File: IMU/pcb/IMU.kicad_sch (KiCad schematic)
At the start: 1 part, among them J2 Conn_01x10_Socket

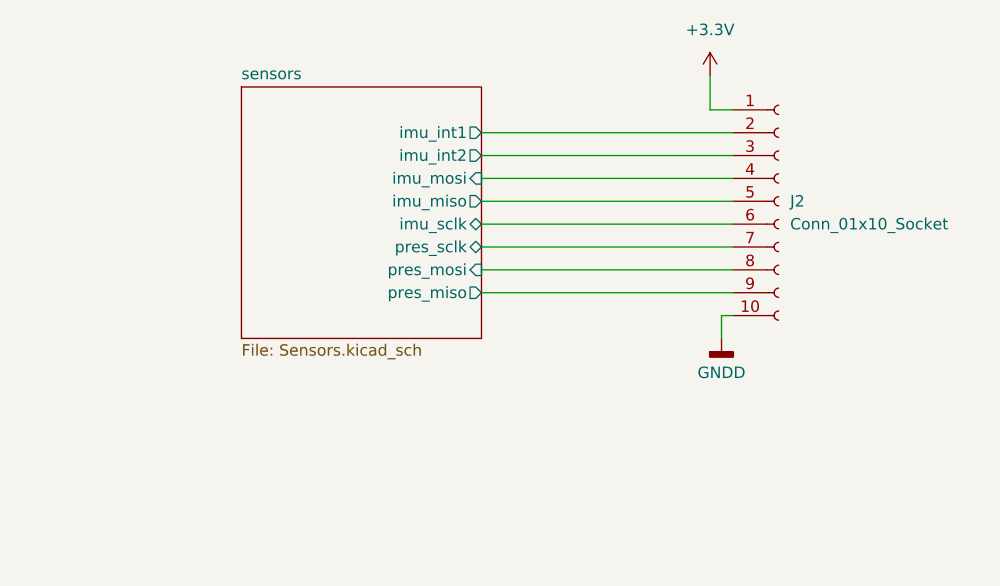
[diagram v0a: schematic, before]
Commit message: Finished IMU Rev 1
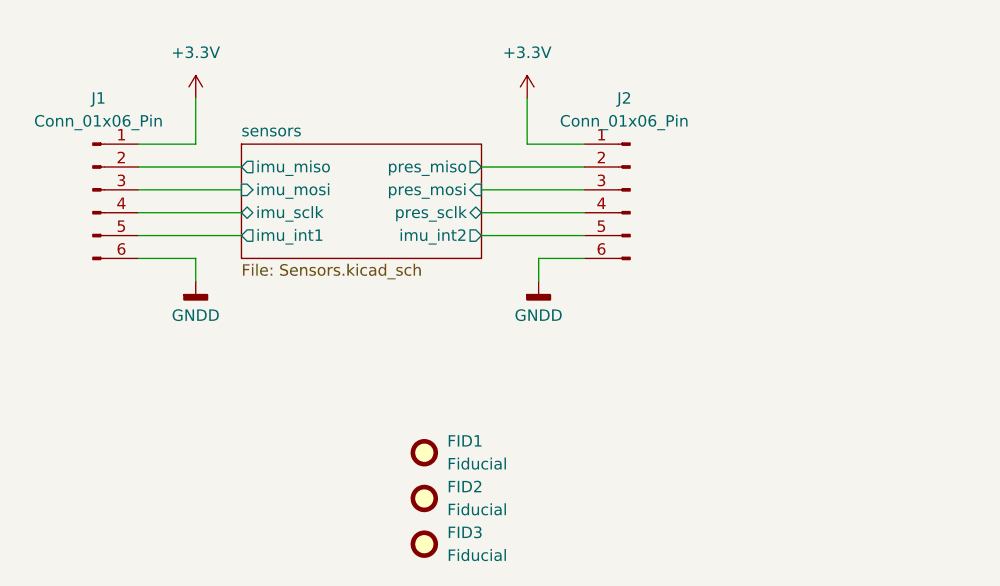
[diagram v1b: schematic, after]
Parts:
- removed J2: Conn_01x10_Socket, Connector_PinHeader_2.54mm:PinHeader_1x10_P2.54mm_Vertical, symbol Connector:Conn_01x10_Socket
- added FID1, FID2, FID3: Fiducial, Fiducial:Fiducial_1mm_Mask2mm, symbol Mechanical:Fiducial
- added J1, J2: Conn_01x06_Pin, Connector_PinHeader_2.54mm:PinHeader_1x06_P2.54mm_Vertical, symbol Connector:Conn_01x06_Pin
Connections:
- net +3.3V: now also J1.1 (Pin_1), J2.1 (Pin_1)
- net GNDD: now also J1.6 (Pin_6), J2.6 (Pin_6)
- net sensors/imu_int1: now also J1.5 (Pin_5)
- net sensors/imu_int2: now also J2.5 (Pin_5)
- net sensors/imu_miso: now also J1.2 (Pin_2)
- net sensors/imu_mosi: now also J1.3 (Pin_3)
- net sensors/imu_sclk: now also J1.4 (Pin_4)
- net sensors/pres_miso: now also J2.2 (Pin_2)
- net sensors/pres_mosi: now also J2.3 (Pin_3)
- net sensors/pres_sclk: now also J2.4 (Pin_4)
